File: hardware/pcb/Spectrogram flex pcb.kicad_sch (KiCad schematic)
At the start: 10 parts

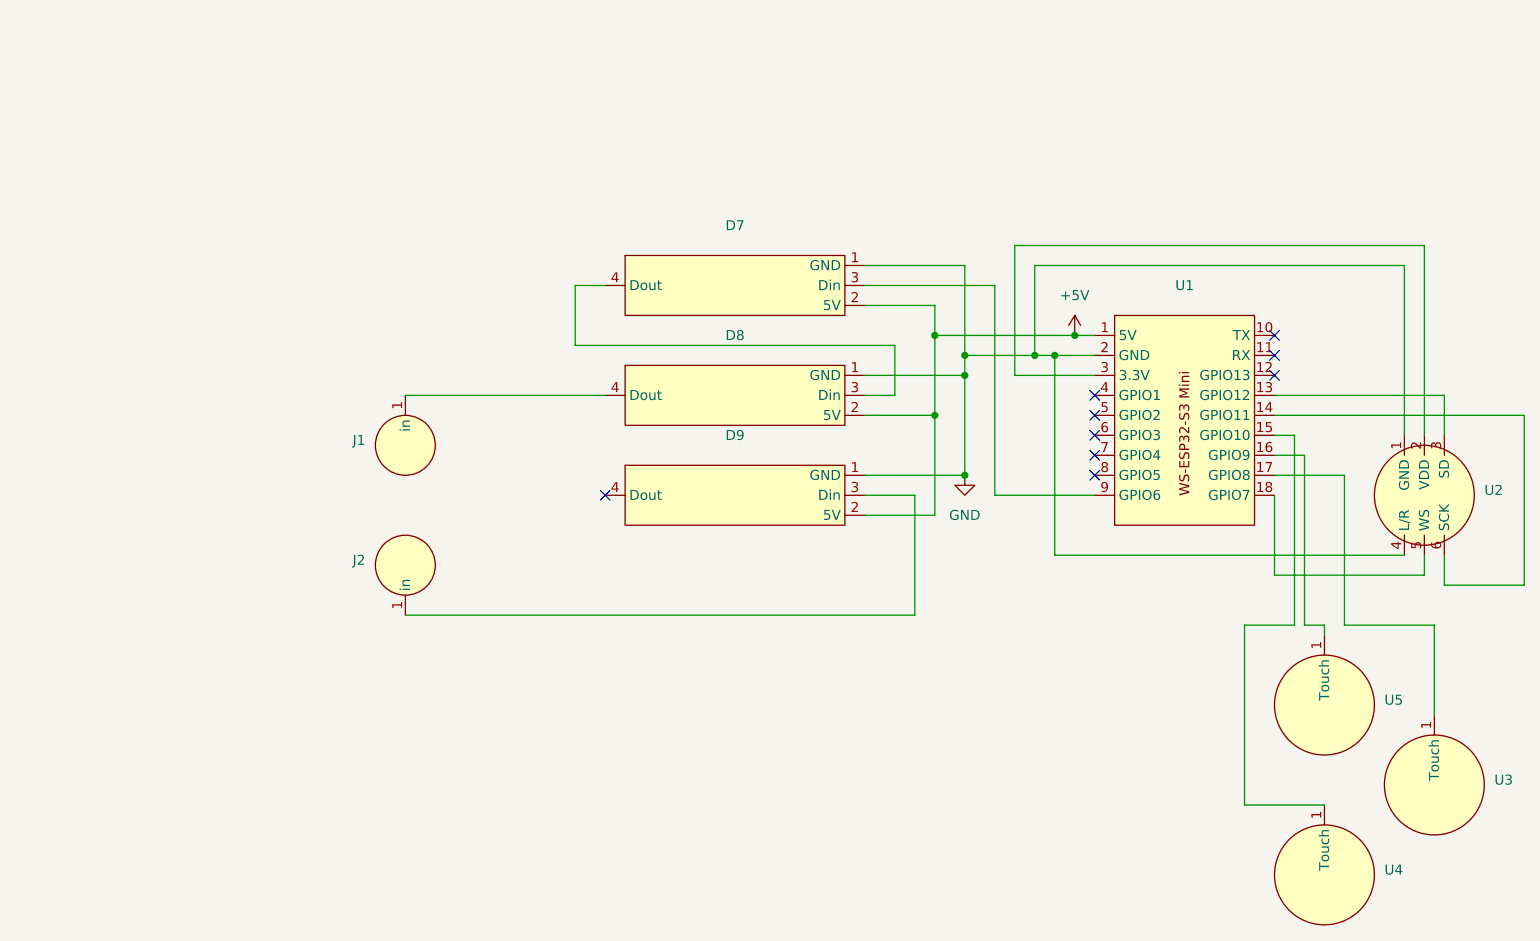
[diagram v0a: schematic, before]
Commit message: PCB revision
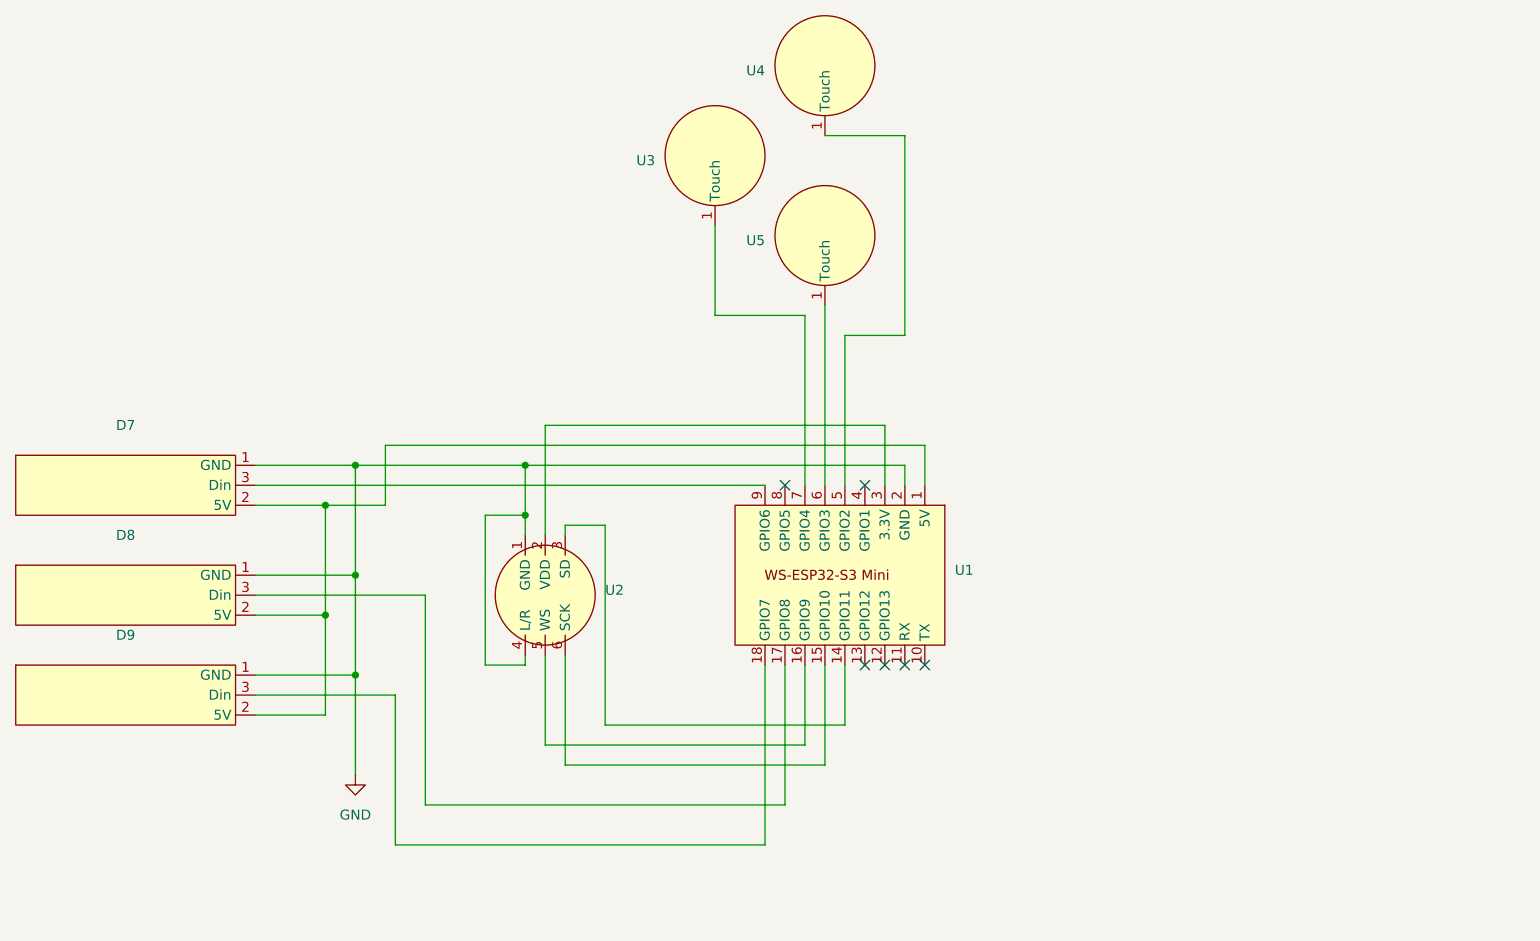
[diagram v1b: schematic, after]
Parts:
- removed J1, J2: ~, Waveshare_ESP32_S3_mini:jumper pad, symbol Waveshare_ESP32_S3_miniDev:JumperPad
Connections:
- net at D8.3 (Din): now also U1.17 (GPIO8); no longer D7.4 (Dout)
- net at D9.3 (Din): now also U1.18 (GPIO7)
- net at U4.1 (Touch): now also U1.5 (GPIO2); no longer U1.15 (GPIO10)
- net at U3.1 (Touch): now also U1.7 (GPIO4); no longer U1.17 (GPIO8)
- net at U5.1 (Touch): now also U1.6 (GPIO3); no longer U1.16 (GPIO9)
- net at U1.13 (GPIO12): no longer U2.3 (SD)
- net at U1.14 (GPIO11): now also U2.3 (SD); no longer U2.6 (SCK)
- net at U2.5 (WS): now also U1.16 (GPIO9); no longer U1.18 (GPIO7)
- net +5V: no longer names the net of D7.2 (5V), D8.2 (5V), D9.2 (5V), U1.1 (5V)
- new net: U1.15 (GPIO10), U2.6 (SCK)
- no-connect marks 9 -> 6
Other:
- moved on the sheet: U1, U2, U3, U4, U5
